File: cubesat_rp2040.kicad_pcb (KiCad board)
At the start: 4 copper layers, 90.2 x 95.9 mm, 79 parts, among them J301 USB_C_Receptacle_USB2.0, J401 FTSH-105-01-L-DV-007, J701 Conn_01x02, SW901 SW_Push, U1001 TUSB4041I, U201 L7983, U501 RP2040, U701 W25Q128JVS, U801 T6405 R24M0

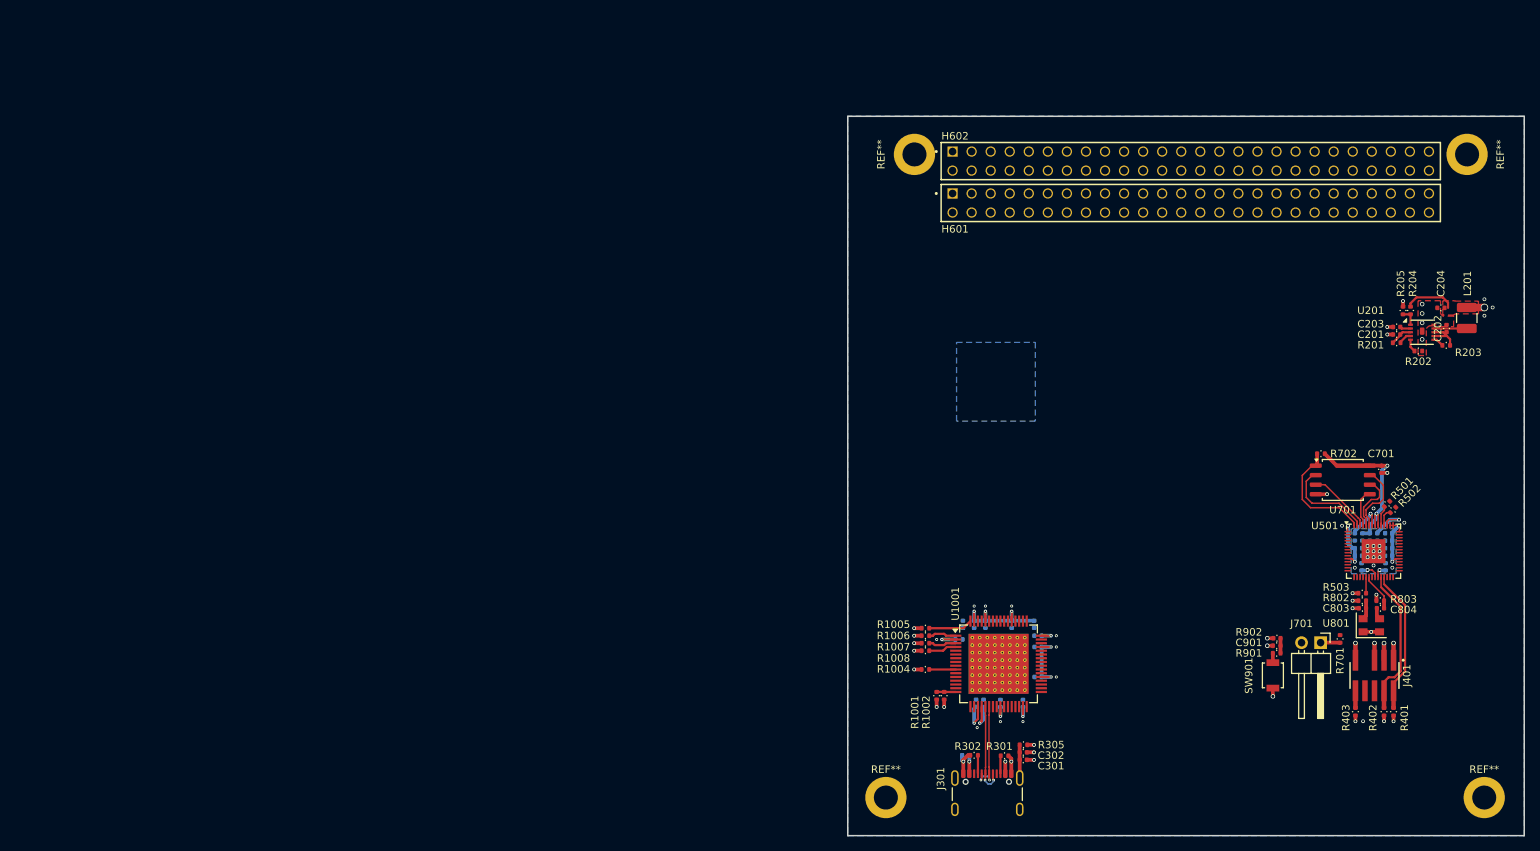
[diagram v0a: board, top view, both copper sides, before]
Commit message: Major update, everything has been touched
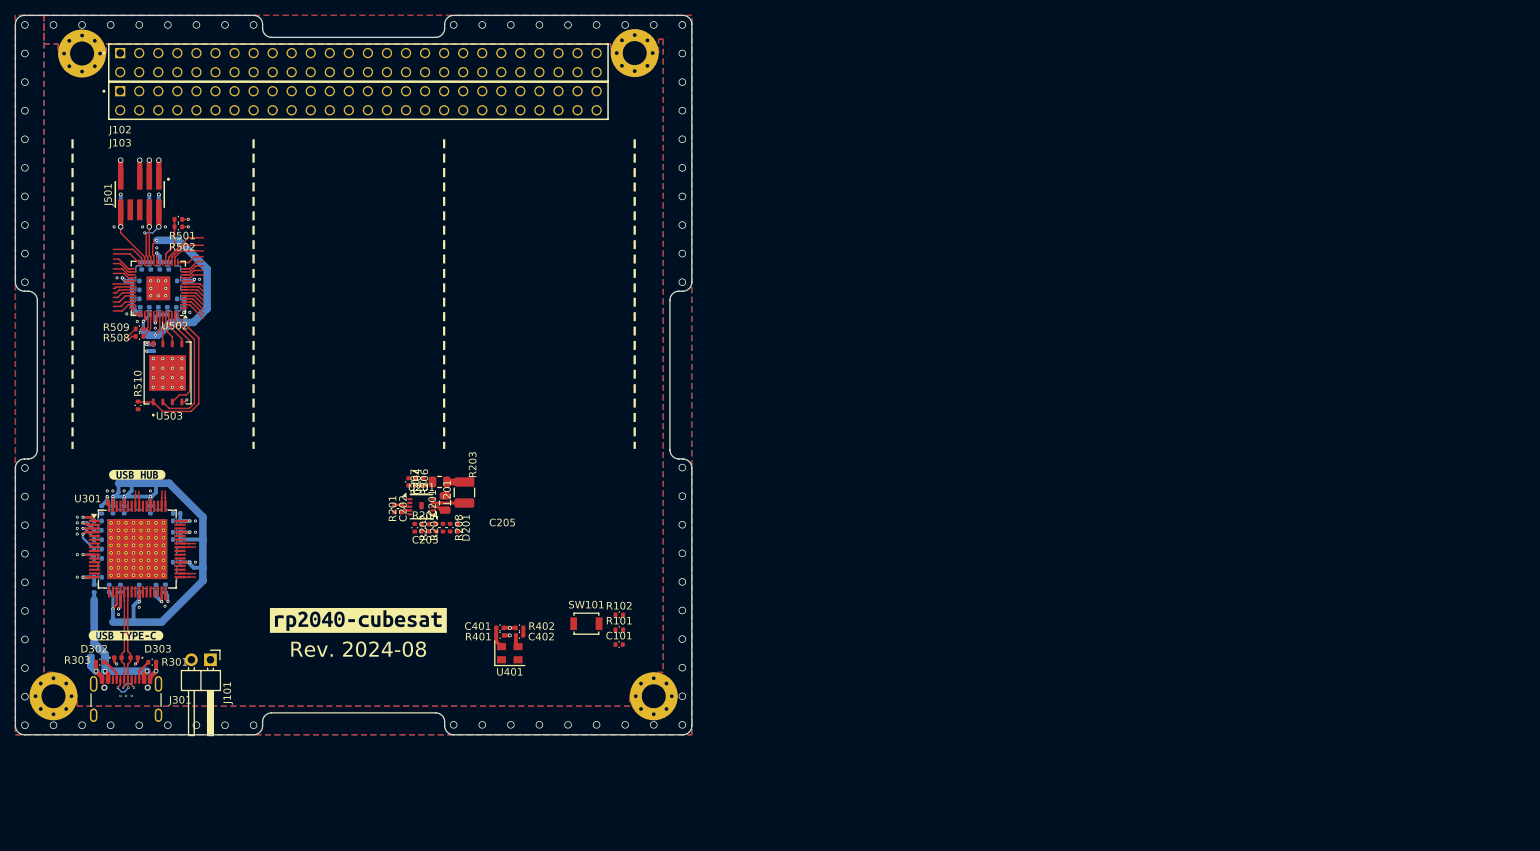
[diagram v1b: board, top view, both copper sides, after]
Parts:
- removed C1001, C1002, C1003, C1004, C1005, C1006, C1007, C1008, C1009, C1010, C1011, C301, C803: 100n, cubesat_rp2040:C_0402_1005Metric
- removed C1012, C1013: 1u, cubesat_rp2040:C_0402_1005Metric
- removed C302: 1n, cubesat_rp2040:C_0402_1005Metric
- removed C303: 10u, cubesat_rp2040:C_0402_1005Metric
- removed C701: C_Small, cubesat_rp2040:C_0402_1005Metric
- removed C804: 10n, cubesat_rp2040:C_0402_1005Metric
- removed C901: C, cubesat_rp2040:C_0402_1005Metric
- removed H601, H602: ESQ-126-39-G-D, cubesat_rp2040:SAMTEC_ESQ-126-39-G-D
- removed J401: FTSH-105-01-L-DV-007, cubesat_rp2040:SAMTEC_FTSH-105-01-L-DV-007
- removed J701: Conn_01x02, Connector_PinHeader_2.54mm:PinHeader_1x02_P2.54mm_Horizontal
- removed R1001: 90.9k 1%, cubesat_rp2040:R_0402_1005Metric
- removed R1002: 10k 1%, cubesat_rp2040:R_0402_1005Metric
- removed R1004, R1005, R1006, R1007, R1008: 4.7k, cubesat_rp2040:R_0402_1005Metric
- removed R302: 5.1k 10%, cubesat_rp2040:R_0402_1005Metric
- removed R403, R901, R902: R, cubesat_rp2040:R_0402_1005Metric
- removed R503: 0R, cubesat_rp2040:R_0402_1005Metric
- removed R701: 1k, cubesat_rp2040:R_0402_1005Metric
- removed R702, R803: 10k, cubesat_rp2040:R_0402_1005Metric
- removed R802: 33R, cubesat_rp2040:R_0402_1005Metric
- removed REF** (x4): MountingHole_3.2mm_M3_ISO14580_Pad, MountingHole:MountingHole_3.2mm_M3_ISO14580_Pad
- removed SW901: SW_Push, Button_Switch_SMD:SW_SPST_B3U-1000P
- removed U1001: TUSB4041I, Package_QFP:HTQFP-64-1EP_10x10mm_P0.5mm_EP8x8mm_Mask4.4x4.4mm_ThermalVias
- removed U501: RP2040, Package_DFN_QFN:QFN-56-1EP_7x7mm_P0.4mm_EP3.2x3.2mm
- removed U701: W25Q128JVS, Package_SO:SOIC-8_5.23x5.23mm_P1.27mm
- removed U801: T6405 R24M0, cubesat_rp2040:Crystal_SMD_Rakon_3225-4Pin_3.2x2.5mm
- added C101: 100n, cubesat_rp2040:C_0402_1005Metric, F.Cu at (121.9, 126.9)
- added C205: 1u, Capacitor_SMD:C_0805_2012Metric, F.Cu at (98.0, 105.3)
- added C206: 10u, Capacitor_SMD:C_0805_2012Metric, B.Cu at (52.5, 128.9)
- added C304: 1u, cubesat_rp2040:C_0402_1005Metric, B.Cu at (63.0, 112.9)
- added C305: 1u, cubesat_rp2040:C_0402_1005Metric, B.Cu at (63.0, 109.5)
- added C306: 100n, cubesat_rp2040:C_0402_1005Metric, B.Cu at (54.0, 119.5)
- added C307: 100n, cubesat_rp2040:C_0402_1005Metric, B.Cu at (63.0, 116.0)
- added C308: 100n, cubesat_rp2040:C_0402_1005Metric, B.Cu at (54.5, 109.0)
- added C309: 100n, cubesat_rp2040:C_0402_1005Metric, B.Cu at (63.0, 112.0)
- added C310: 100n, cubesat_rp2040:C_0402_1005Metric, B.Cu at (58.0, 119.5)
- added C311: 100n, cubesat_rp2040:C_0402_1005Metric, B.Cu at (59.5, 109.0)
- added C312: 100n, cubesat_rp2040:C_0402_1005Metric, B.Cu at (56.0, 109.0)
- added C313: 100n, cubesat_rp2040:C_0402_1005Metric, B.Cu at (60.2, 119.5)
- added C314: 100n, cubesat_rp2040:C_0402_1005Metric, B.Cu at (63.0, 110.5)
- added C315: 100n, cubesat_rp2040:C_0402_1005Metric, B.Cu at (52.5, 111.7)
- added C316: 100n, cubesat_rp2040:C_0402_1005Metric, B.Cu at (55.5, 119.5)
- added C401: 100n, cubesat_rp2040:C_0402_1005Metric, F.Cu at (106.0, 124.7)
- added C402: 10n, cubesat_rp2040:C_0402_1005Metric, F.Cu at (108.7, 125.7)
- added C513: 100n, cubesat_rp2040:C_0402_1005Metric, B.Cu at (63.5, 80.9)
- added C514: 100n, cubesat_rp2040:C_0402_1005Metric, B.Cu at (58.1, 82.5)
- added C515: 100n, cubesat_rp2040:C_0402_1005Metric, B.Cu at (60.7, 76.5)
- added D201: GREEN, LED_SMD:LED_0402_1005Metric, F.Cu at (100.4, 111.4)
- added D302: D_TVS, Diode_SMD:D_0402_1005Metric, F.Cu at (55.1, 128.7)
- added D303: D_TVS, Diode_SMD:D_0402_1005Metric, F.Cu at (57.3, 128.7)
- added H101: MountingHole_Pad, MountingHole:MountingHole_3.2mm_M3_Pad_Via, F.Cu at (46.5, 133.8)
- added H102: MountingHole_Pad, MountingHole:MountingHole_3.2mm_M3_Pad_Via, F.Cu at (126.5, 133.8)
- added H103: MountingHole_Pad, MountingHole:MountingHole_3.2mm_M3_Pad_Via, F.Cu at (124.0, 48.1)
- added H104: MountingHole_Pad, MountingHole:MountingHole_3.2mm_M3_Pad_Via, F.Cu at (50.3, 48.1)
- added J101: Conn_01x02, Connector_PinHeader_2.54mm:PinHeader_1x02_P2.54mm_Horizontal, F.Cu at (67.5, 129.0)
- added J102: ESQ-126-39-G-D, cubesat_rp2040:SAMTEC_ESQ-126-39-G-D, F.Cu at (55.4, 48.1)
- added J103: ESQ-126-39-G-D, cubesat_rp2040:SAMTEC_ESQ-126-39-G-D, F.Cu at (55.4, 53.2)
- added J501: FTSH-105-01-L-DV-007, cubesat_rp2040:SAMTEC_FTSH-105-01-L-DV-007, F.Cu at (58.0, 66.9)
- added R101: 100k, cubesat_rp2040:R_0402_1005Metric, F.Cu at (121.9, 125.0)
- added R102: 10k, cubesat_rp2040:R_0402_1005Metric, F.Cu at (121.9, 123.0)
- added R206: 47k, cubesat_rp2040:R_0402_1005Metric, F.Cu at (94.8, 105.3)
- added R207: 16k, cubesat_rp2040:R_0402_1005Metric, F.Cu at (95.8, 105.3)
- added R208: 470R, cubesat_rp2040:R_0402_1005Metric, F.Cu at (99.4, 111.3)
- added R303: 5.1k 10%, cubesat_rp2040:R_0402_1005Metric, F.Cu at (52.7, 129.3)
- added R304: 90.9k 1%, cubesat_rp2040:R_0402_1005Metric, B.Cu at (52.0, 119.5)
- added R306: 9.53k 1%, cubesat_rp2040:R_0402_1005Metric, B.Cu at (61.5, 119.5)
- added R307: 4.7k, cubesat_rp2040:R_0402_1005Metric, B.Cu at (52.5, 115.5)
- added R308: 4.7k, cubesat_rp2040:R_0402_1005Metric, B.Cu at (53.0, 109.0)
- added R309: 4.7k, cubesat_rp2040:R_0402_1005Metric, B.Cu at (52.5, 110.5)
- added R310: 4.7k, cubesat_rp2040:R_0402_1005Metric, B.Cu at (52.5, 113.0)
- added R311: 4.7k, cubesat_rp2040:R_0402_1005Metric, B.Cu at (52.5, 114.2)
- added R505: 100k, cubesat_rp2040:R_0402_1005Metric, B.Cu at (60.6, 69.0)
- added R506: 100k, cubesat_rp2040:R_0402_1005Metric, B.Cu at (59.3, 69.0)
- added R507: 100k, cubesat_rp2040:R_0402_1005Metric, B.Cu at (55.5, 69.0)
- added R508: 27R, cubesat_rp2040:R_0402_1005Metric, F.Cu at (58.0, 85.9)
- added R509: 27R, cubesat_rp2040:R_0402_1005Metric, F.Cu at (58.0, 84.9)
- added R510: 1k, cubesat_rp2040:R_0402_1005Metric, F.Cu at (57.8, 95.0)
- added SW101: SW_Push, Button_Switch_SMD:SW_SPST_B3U-1000P, F.Cu at (117.6, 124.1)
- added U301: TUSB4041I, Package_QFP:HTQFP-64-1EP_10x10mm_P0.5mm_EP8x8mm_Mask4.4x4.4mm_ThermalVias, F.Cu at (57.7, 114.2)
- added U401: T6405 R24M0, cubesat_rp2040:Crystal_SMD_Rakon_3225-4Pin_3.2x2.5mm, F.Cu at (107.3, 128.1)
- added U502: RP2040, Package_DFN_QFN:QFN-56-1EP_7x7mm_P0.4mm_EP3.2x3.2mm, F.Cu at (60.5, 79.5)
- added U503: S25FL128SAGNFM000, cubesat_rp2040:SON8_S25FL128SAGNFI001_INF, F.Cu at (61.7, 90.7)
- added kibuzzard-66B1EB87: G***, kibuzzard-66B1EB87, F.Cu at (57.7, 104.3)
- added kibuzzard-66B1EBBE: G***, kibuzzard-66B1EBBE, F.Cu at (56.2, 125.7)
- added kibuzzard-66B4F7EF: G***, kibuzzard-66B4F7EF, F.Cu at (87.2, 123.7)
- C201: value 470n -> 1u; footprint cubesat_rp2040:C_0402_1005Metric -> Capacitor_SMD:C_0805_2012Metric
- C202: value 1u -> 470n
- C203: value 100n -> 470n
- C204, C505: value 1u -> 100n
- C502: value 100n -> 1u
- R204: value 47k -> 56k
- R205: value 16k -> 100k
- R305: value 1M -> 10k 1%; moved to B.Cu
- R401: value R -> 33R
- R402: value R -> 10k
- R501, R502: value 27R -> 0R
- moved C509 170.4 mm to (57.5, 78.5), turned to 0 degrees
- moved C508 170.3 mm to (57.5, 79.7), turned to 0 degrees
- moved C507 170.3 mm to (57.5, 80.9), turned to 0 degrees
- moved C502 168.6 mm to (58.3, 76.5)
- moved C501 166.8 mm to (59.9, 87.3), turned to -90 degrees
- moved R502 166.3 mm to (63.2, 71.3), turned to 0 degrees
- moved C505 165.5 mm to (59.5, 76.5), turned to -90 degrees
- moved R501 165.5 mm to (63.2, 70.3), turned to 0 degrees
- moved C506 164.9 mm to (62.9, 82.5), turned to 90 degrees
- moved C504 164.2 mm to (59.3, 82.5), turned to 90 degrees
- moved C512 164.0 mm to (60.5, 82.5)
- moved C503 162.2 mm to (61.9, 76.5)
- moved C510 162.1 mm to (63.5, 78.5), turned to 180 degrees
- moved C511 162.1 mm to (61.7, 82.5), turned to 90 degrees
- moved C202 142.3 mm to (92.0, 108.8), turned to -90 degrees
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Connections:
- net /USB 2.0 Hub/USB_UP.D+ renamed /USB/USB_UP.D+
- net /USB 2.0 Hub/USB_UP.D- renamed /USB/USB_UP.D-
- net /USB Type C connector/USB_UP.CC2 renamed /USB/USB_UP.CC2
- net /VBUS to 3V3/FSW renamed /Power/FSW
- net Net-(U201-LX) renamed /Power/LX
- C201 pad 1: /VBUS to 3V3/VCC -> VBUS
- C202 pad 1: /VBUS -> /Power/VCC
- C203 pad 1: +3V3 -> /Power/EN/UVLO
- C501 pad 1: +1V1 -> +3V3
- C503 pad 1: +1V1 -> +3V3
- C504 pad 1: +3V3 -> +1V1
- C505 pad 1: +3V3 -> +1V1
- C506 pad 1: +3V3 -> +1V1
- J301 pad A4: /USB 2.0 Hub/VBUS -> VBUS
- J301 pad A5: /USB Type C connector/USB_UP.CC1 -> /USB/USB_UP.CC1
- J301 pad A9: /USB 2.0 Hub/VBUS -> VBUS
- J301 pad B4: /USB 2.0 Hub/VBUS -> VBUS
- J301 pad B9: /USB 2.0 Hub/VBUS -> VBUS
- J301 pad S1: Earth -> GND
- R201 pad 2: /VBUS to 3V3/VCC -> /Power/VCC
- R203 pad 1: /VBUS -> /Power/EN/UVLO
- R203 pad 2: /Debug/~{RESET} -> VBUS
- R204 pad 1: +3V3 -> GND
- R204 pad 2: Net-(U201-VOUT/FB) -> /Power/EN/UVLO
- R205 pad 1: Net-(U201-VOUT/FB) -> VBUS
- R205 pad 2: GND -> /RP2040/RUN
- R305 pad 1: Earth -> /USB/USB_VBUS
- R401 pad 1: /Debug/SWDIO -> +3V3
- R401 pad 2: +3V3 -> Net-(U401-VCC)
- R402 pad 1: GND -> /Oscillator/F_{out}
- R402 pad 2: /Debug/SWCLK -> GND
- R501 pad 1: /RP2040/USB.D+ -> /RP2040/TESTEN
- R501 pad 2: Net-(U501-USB_DP) -> +3V3
- R502 pad 1: /RP2040/USB.D- -> /RP2040/TESTEN
- R502 pad 2: Net-(U501-USB_DM) -> GND
- U201 pad 1: Net-(U201-VOUT/FB) -> /Power/FB
- U201 pad 3: /VBUS to 3V3/VCC -> /Power/VCC
- U201 pad 6: /Debug/~{RESET} -> /RP2040/RUN
- U201 pad 7: /VBUS -> /Power/EN/UVLO
- U201 pad 8: /VBUS -> VBUS
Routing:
- net +1V1: track 44.9 -> 114.9 mm
- net /RP2040/QSPI.~{SS}: track 0.00 -> 22.2 mm
- net VBUS: track 0.00 -> 21.1 mm, vias 0 -> 2
- net +3V3: track 70.8 -> 50.6 mm, vias 17 -> 16
- net /Debug/SWCLK: track 20.0 -> 0.00 mm
- net /Debug/SWDIO: track 19.3 -> 0.00 mm
- net /RP2040/QSPI.SD1: track 0.00 -> 17.8 mm
- net /Flash/QSPI.~{SS}: track 15.8 -> 0.00 mm
- net /RP2040/QSPI.SD2: track 0.00 -> 14.2 mm
- net /Flash/QSPI.SD1: track 12.4 -> 0.00 mm
- net GND: track 33.8 -> 22.4 mm, vias 59 -> 137
- net /RP2040/SWDIO: track 0.00 -> 10.4 mm, vias 0 -> 2
- net /RP2040/RUN: track 0.00 -> 10.1 mm, vias 0 -> 1
- net /Flash/QSPI.SD3: track 9.37 -> 0.00 mm
- net /RP2040/SWCLK: track 0.00 -> 8.90 mm, vias 0 -> 1
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- added copper zone on In2.Cu, net +3V3
- removed copper zone on B.Cu, net +3V3
- removed copper zone on F.Cu, net +3V3
- removed copper zone on In2.Cu, net GND
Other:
- outline, holes or cut-outs redrawn
- board text added: "0"
- board text added: "0 mm"
- board text added: "0.0000 mm / 0.0000 mm"
- board text added: "0.01 mm"
- board text added: "0.0152 mm"
- board text added: "0.017"
- board text added: "0.02"
- board text added: "0.035 mm"
- board text added: "0.0994 mm"
- board text added: "0.3000 mm"
- board text added: "1"
- board text added: "1.265 mm"
- board text added: "1.5842 mm"
- board text added: "3.3"
- board text added: "4"
- board text added: "4.1"
- board text added: "4.6"
- board text added: "90.1700 mm x 95.8900 mm"
- board text added: "B.Cu"
- board text added: "B.Mask"
- board text added: "B.Paste"
- board text added: "B.Silkscreen"
- board text added: "BOARD CHARACTERISTICS"
- board text added: "Board Thickness:"
- board text added: "Board overall dimensions:"
- board text added: "Bottom Silk Screen"
- board text added: "Bottom Solder Mask"
- board text added: "Bottom Solder Paste"
- board text added: "Castellated pads:"
- board text added: "Color"
- board text added: "Copper Finish:"
- board text added: "Copper Layer Count:"
- board text added: "Dielectric 1"
- board text added: "Dielectric 2"
- board text added: "Dielectric 3"
- board text added: "ENIG"
- board text added: "Edge card connectors:"
- board text added: "Epsilon R"
- board text added: "F.Cu"
- board text added: "F.Mask"
- board text added: "F.Paste"
- board text added: "F.Silkscreen"
- board text added: "FR4"
- board text added: "FR4 natural"
- board text added: "Green"
- board text added: "Impedance Control:"
- board text added: "In1.Cu"
- board text added: "In2.Cu"
- board text added: "Layer Name"
- board text added: "Loss Tangent"
- board text added: "Material"
- board text added: "Min hole diameter:"
- board text added: "Min track/spacing:"
- board text added: "No"
- board text added: "Not specified"
- board text added: "Plated Board Edge:"
- board text added: "Rev. ${REVISION}"
- board text added: "Thickness (mm)"
- board text added: "Top Silk Screen"
- board text added: "Top Solder Mask"
- board text added: "Top Solder Paste"
- board text added: "Type"
- board text added: "White"
- board text added: "Yes"
- board text added: "copper"
- board text added: "core"
- board text added: "prepreg"
